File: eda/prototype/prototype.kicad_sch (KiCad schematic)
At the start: 9 parts, among them U1 8088_Min_Mode, U2 GAL16V8, U3 74HC161, U4 74HC574, U5 SST39SF040, U6 HM62256BLP, U7 HM62256BLP, U8 74HC245, X1 CXO_DIP8

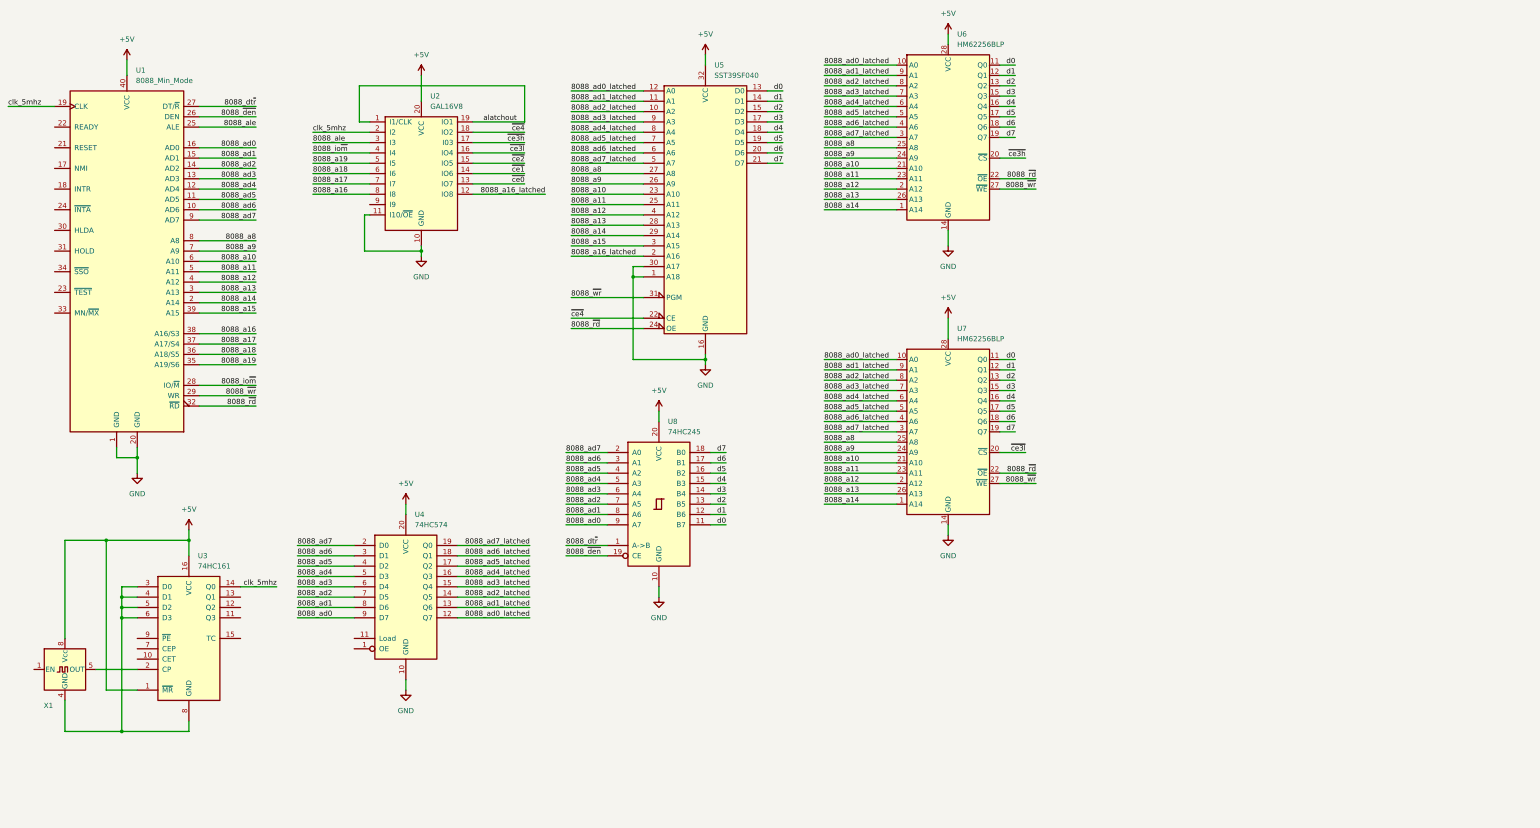
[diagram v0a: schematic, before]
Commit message: eda: prototype: bit more filling out
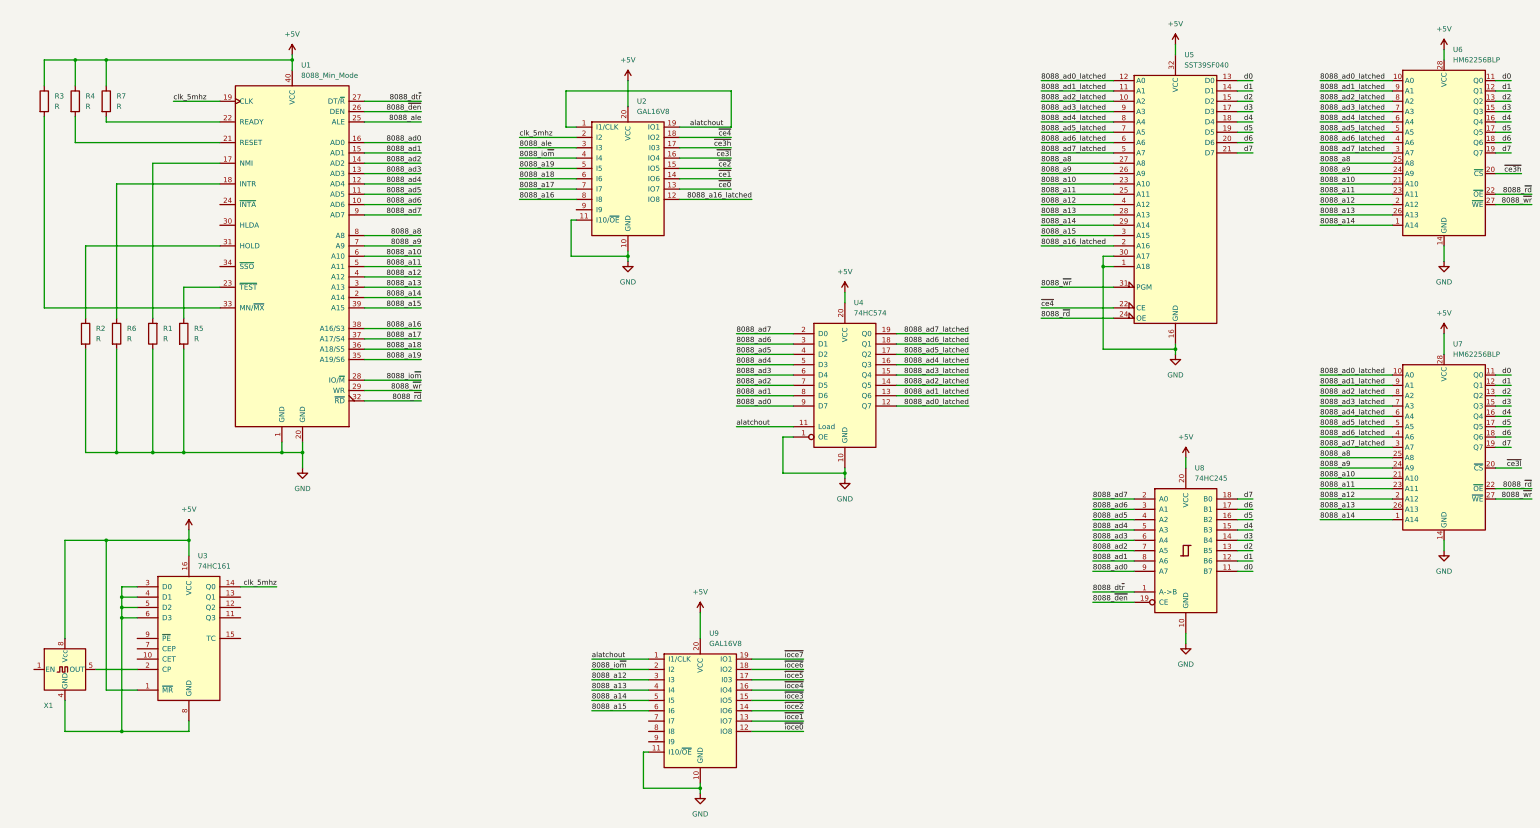
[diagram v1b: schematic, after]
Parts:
- added R1, R2, R3, R4, R5, R6, R7: R, symbol Device:R
- added U9: GAL16V8, symbol Logic_Programmable:GAL16V8
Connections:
- net +5V: now also R3.1, R4.1, R7.1, U9.20 (VCC)
- net 8088_a12: now also U9.3 (I3)
- net 8088_a13: now also U9.4 (I4)
- net 8088_a14: now also U9.5 (I5)
- net 8088_a15: now also U9.6 (I6)
- net 8088_io~{m}: now also U9.2 (I2)
- net GND: now also U4.1 (OE), R1.1, R2.2, R5.2, R6.2, U9.10 (GND), U9.11 (I10/~{OE})
- net alatchout: now also U4.11 (Load), U9.1 (I1/CLK)
- net at U1.17 (NMI): now also R1.2
- net at U1.18 (INTR): now also R6.1
- net at U1.21 (RESET): now also R4.2
- net at U1.22 (READY): now also R7.2
- net at U1.23 (~{TEST}): now also R5.1
- net at U1.31 (HOLD): now also R2.1
- net at U1.33 (MN/~{MX}): now also R3.2
- new net ~{ioce0}: U9.12 (IO8)
- new net ~{ioce1}: U9.13 (IO7)
- new net ~{ioce2}: U9.14 (IO6)
- new net ~{ioce3}: U9.15 (IO5)
- new net ~{ioce4}: U9.16 (IO4)
- new net ~{ioce5}: U9.17 (I03)
- new net ~{ioce6}: U9.18 (IO2)
- new net ~{ioce7}: U9.19 (IO1)
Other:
- moved on the sheet: U1, U2, U4, U5, U6, U7, U8
